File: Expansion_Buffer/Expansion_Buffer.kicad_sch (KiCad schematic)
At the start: 18 parts, among them J1 Out, J4 In

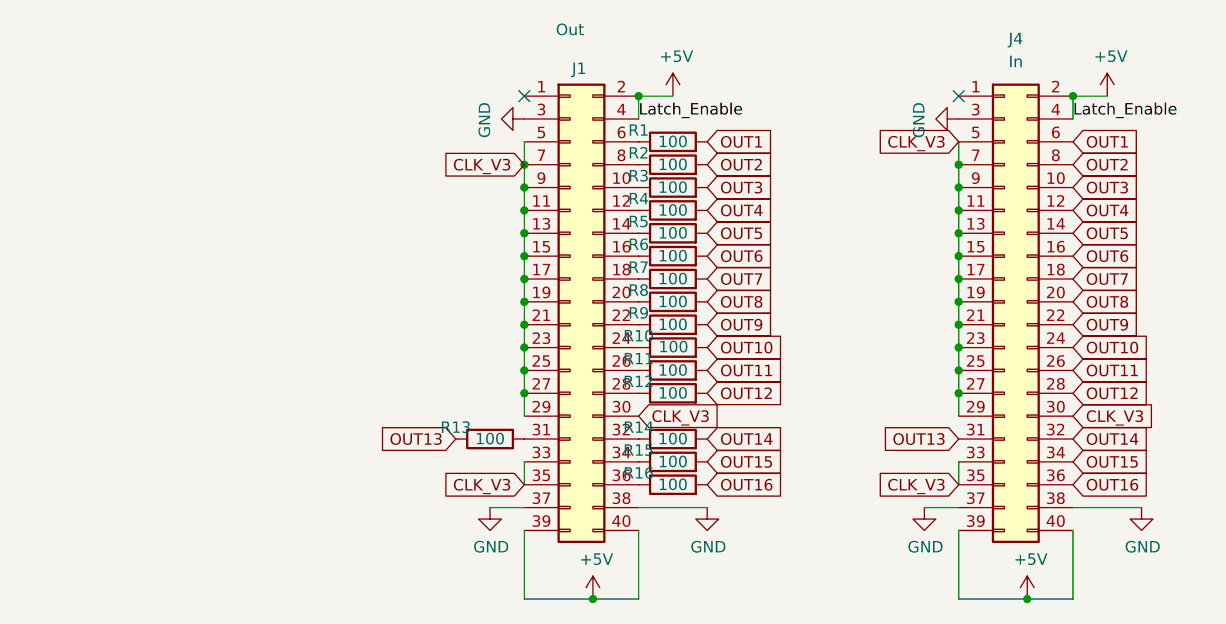
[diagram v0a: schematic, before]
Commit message: added gerbers
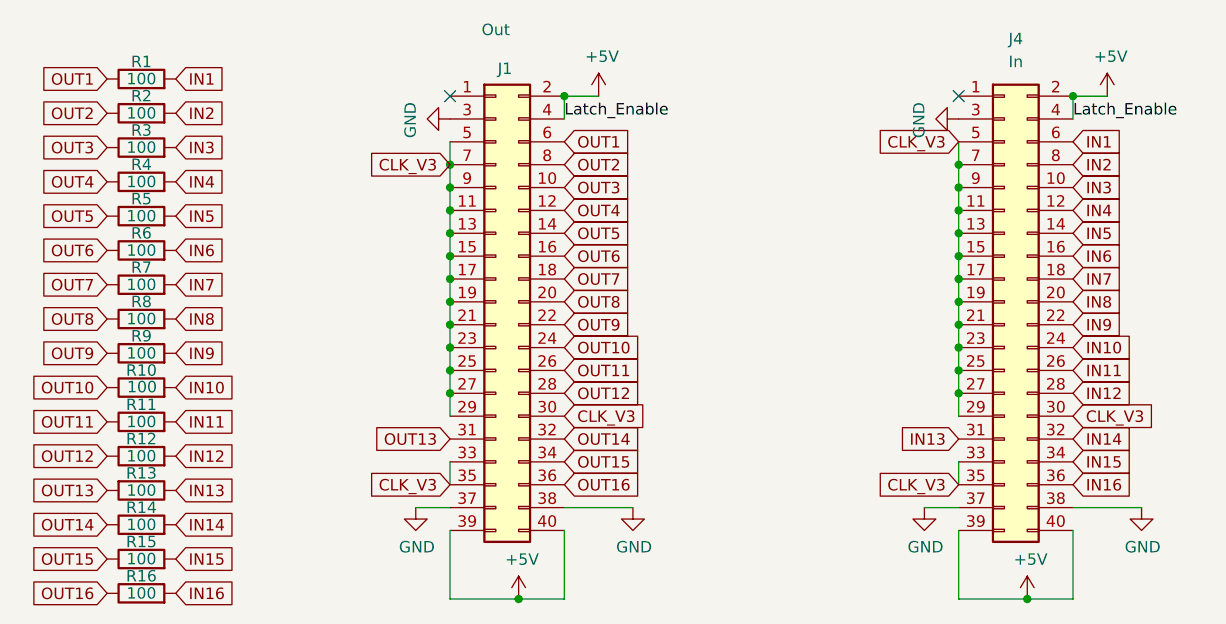
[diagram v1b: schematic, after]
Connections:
- net OUT1: now also J1.6 (Pin_6), R1.1; no longer J4.6 (Pin_6), R1.2
- net OUT10: now also J1.24 (Pin_24), R10.1; no longer J4.24 (Pin_24), R10.2
- net OUT11: now also J1.26 (Pin_26), R11.1; no longer J4.26 (Pin_26), R11.2
- net OUT12: now also J1.28 (Pin_28), R12.1; no longer J4.28 (Pin_28), R12.2
- net OUT13: now also J1.31 (Pin_31), R13.2; no longer J4.31 (Pin_31), R13.1
- net OUT14: now also J1.32 (Pin_32), R14.1; no longer J4.32 (Pin_32), R14.2
- net OUT15: now also J1.34 (Pin_34), R15.1; no longer J4.34 (Pin_34), R15.2
- net OUT16: now also J1.36 (Pin_36), R16.1; no longer J4.36 (Pin_36), R16.2
- net OUT2: now also J1.8 (Pin_8), R2.1; no longer J4.8 (Pin_8), R2.2
- net OUT3: now also J1.10 (Pin_10), R3.1; no longer J4.10 (Pin_10), R3.2
- net OUT4: now also J1.12 (Pin_12), R4.1; no longer J4.12 (Pin_12), R4.2
- net OUT5: now also J1.14 (Pin_14), R5.1; no longer J4.14 (Pin_14), R5.2
- net OUT6: now also J1.16 (Pin_16), R6.1; no longer J4.16 (Pin_16), R6.2
- net OUT7: now also J1.18 (Pin_18), R7.1; no longer J4.18 (Pin_18), R7.2
- net OUT8: now also J1.20 (Pin_20), R8.1; no longer J4.20 (Pin_20), R8.2
- net OUT9: now also J1.22 (Pin_22), R9.1; no longer J4.22 (Pin_22), R9.2
- new net IN1: J4.6 (Pin_6), R1.2
- new net IN10: J4.24 (Pin_24), R10.2
- new net IN11: J4.26 (Pin_26), R11.2
- new net IN12: J4.28 (Pin_28), R12.2
- new net IN13: J4.31 (Pin_31), R13.1
- new net IN14: J4.32 (Pin_32), R14.2
- new net IN15: J4.34 (Pin_34), R15.2
- new net IN16: J4.36 (Pin_36), R16.2
- new net IN2: J4.8 (Pin_8), R2.2
- new net IN3: J4.10 (Pin_10), R3.2
- new net IN4: J4.12 (Pin_12), R4.2
- new net IN5: J4.14 (Pin_14), R5.2
- new net IN6: J4.16 (Pin_16), R6.2
- new net IN7: J4.18 (Pin_18), R7.2
- new net IN8: J4.20 (Pin_20), R8.2
- new net IN9: J4.22 (Pin_22), R9.2
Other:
- moved on the sheet: J1, R1, R10, R11, R12, R14, R15, R16, R2, R3, R4, R5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
